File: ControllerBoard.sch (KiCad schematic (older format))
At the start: 1 part, among them U1 nice_nano

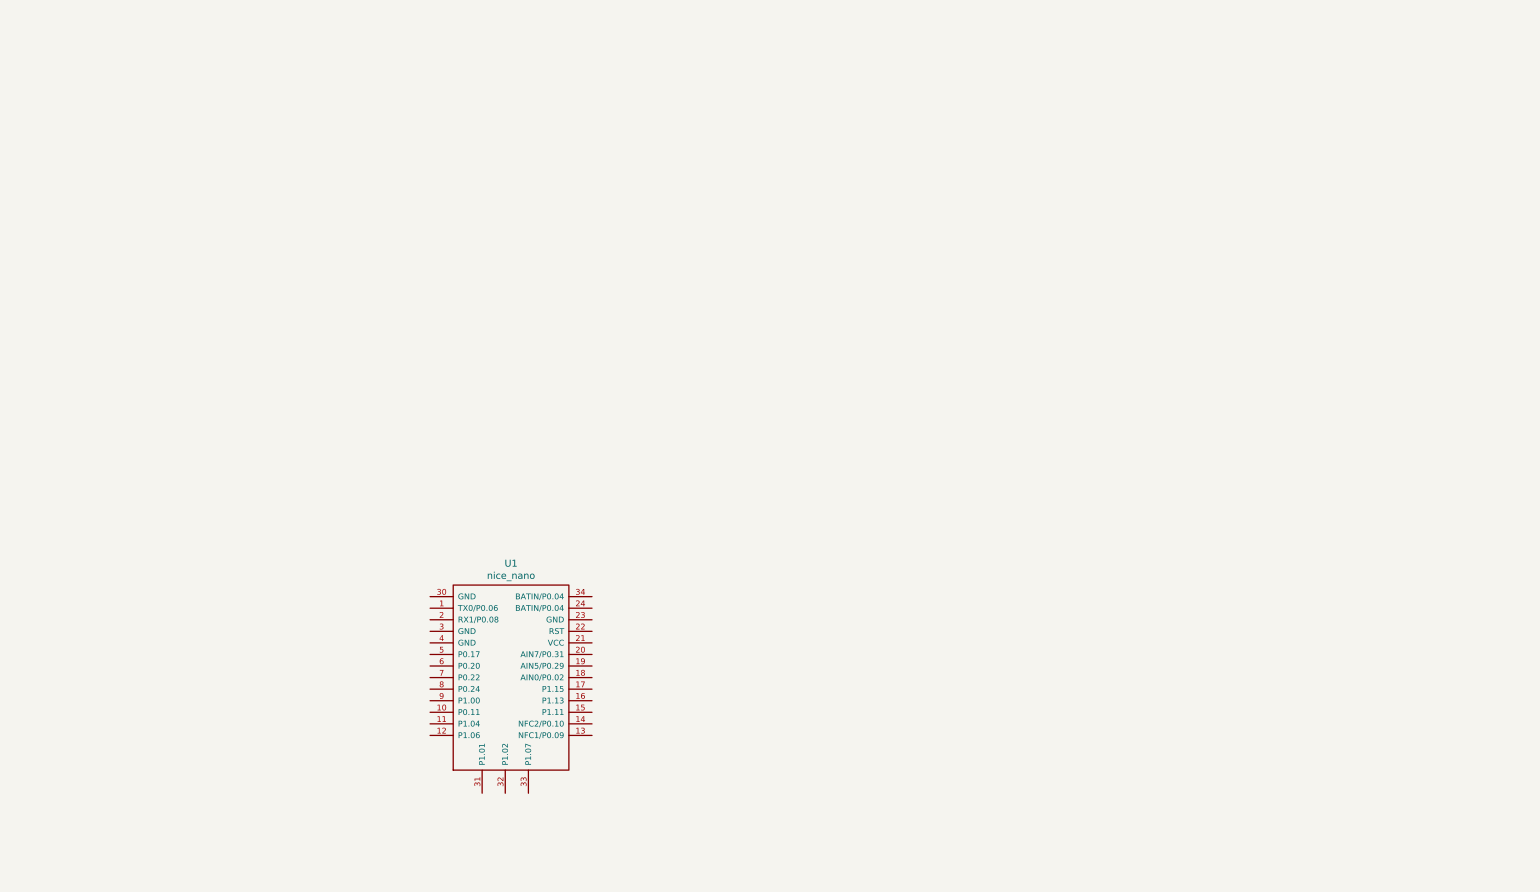
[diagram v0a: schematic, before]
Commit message: First Pass at Wiring
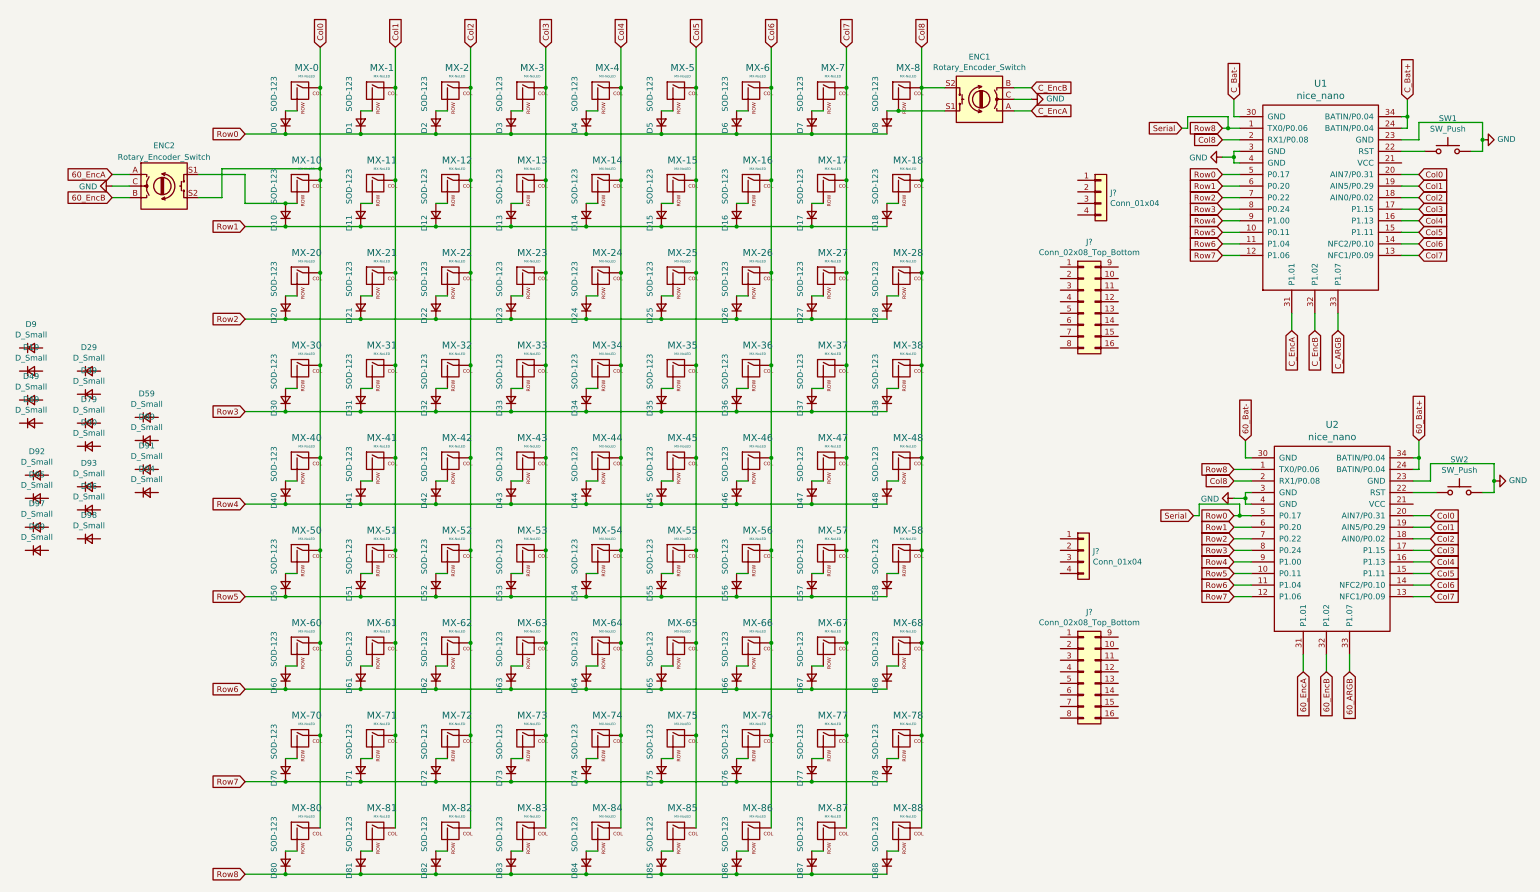
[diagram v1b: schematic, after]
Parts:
- added D0, D1, D10, D11, D12, D13, D14, D15, D16, D17, D18, D2, D20, D21, D22, D23, D24, D25, D26, D27, D28, D3, D30, D31, D32, D33, D34, D35, D36, D37, D38, D4, D40, D41, D42, D43, D44, D45, D46, D47, D48, D5, D50, D51, D52, D53, D54, D55, D56, D57, D58, D6, D60, D61, D62, D63, D64, D65, D66, D67, D68, D7, D70, D71, D72, D73, D74, D75, D76, D77, D78, D8, D80, D81, D82, D83, D84, D85, D86, D87, D88: SOD-123, Keebio-Parts:Diode-Hybrid-Back, symbol Device:D_Small
- added D19, D29, D39, D49, D59, D69, D79, D89, D9, D90, D91, D92, D93, D94, D95, D96, D97, D98, D99: D_Small, symbol Device:D_Small
- added ENC1, ENC2: Rotary_Encoder_Switch, Keebio-Parts:RotaryEncoder_EC11, symbol Device:Rotary_Encoder_Switch
- added J? (x2): Conn_02x08_Top_Bottom, symbol Connector_Generic:Conn_02x08_Top_Bottom
- added J? (x2): Conn_01x04, symbol Connector_Generic:Conn_01x04
- added MX-0, MX-1, MX-10, MX-11, MX-12, MX-13, MX-14, MX-15, MX-16, MX-17, MX-18, MX-2, MX-21, MX-22, MX-23, MX-24, MX-25, MX-26, MX-27, MX-28, MX-3, MX-31, MX-32, MX-33, MX-34, MX-35, MX-36, MX-37, MX-38, MX-4, MX-41, MX-42, MX-43, MX-44, MX-45, MX-46, MX-47, MX-48, MX-5, MX-57, MX-58, MX-6, MX-60, MX-61, MX-62, MX-63, MX-64, MX-65, MX-66, MX-67, MX-68, MX-7, MX-70, MX-71, MX-72, MX-73, MX-74, MX-75, MX-76, MX-77, MX-78, MX-8, MX-80, MX-81, MX-82, MX-83, MX-84, MX-85, MX-86, MX-87, MX-88: MX-NoLED, MX_Alps_Hybrid:MX-1U-NoLED, symbol MX_Alps_Hybrid:MX-NoLED
- added MX-20: MX-NoLED, MX_Alps_Hybrid:MX-1.5U-NoLED, symbol MX_Alps_Hybrid:MX-NoLED
- added MX-30: MX-NoLED, MX_Alps_Hybrid:MX-1.75U-NoLED, symbol MX_Alps_Hybrid:MX-NoLED
- added MX-40: MX-NoLED, MX_Alps_Hybrid:MX-2.25U-NoLED, symbol MX_Alps_Hybrid:MX-NoLED
- added MX-50, MX-51, MX-52, MX-54, MX-55, MX-56: MX-NoLED, MX_Alps_Hybrid:MX-1.25U-NoLED, symbol MX_Alps_Hybrid:MX-NoLED
- added MX-53: MX-NoLED, MX_Alps_Hybrid:MX-6.25U-NoLED, symbol MX_Alps_Hybrid:MX-NoLED
- added SW1, SW2: SW_Push, random-keyboard-parts:SKQG-1155865, symbol Switch:SW_Push
- added U2: nice_nano, nice-nano-kicad:nice_nano, symbol nice_nano:nice_nano
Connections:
- net Row0: now reaches U1.1 (TX0/P0.06)
- net Row0: now also U1.5 (P0.17), D0.1 (K), D1.1 (K), D2.1 (K), D3.1 (K), D4.1 (K), D5.1 (K), D6.1 (K), D7.1 (K), D8.1 (K), D80.1 (K), D81.1 (K), D82.1 (K), D83.1 (K), D84.1 (K), D85.1 (K), D86.1 (K), D87.1 (K), D88.1 (K), U2.1 (TX0/P0.06), U2.5 (P0.17)
- net Row5: now reaches U1.10 (P0.11)
- net Row5: now also D50.1 (K), D51.1 (K), D52.1 (K), D53.1 (K), D54.1 (K), D55.1 (K), D56.1 (K), D57.1 (K), D58.1 (K), U2.10 (P0.11)
- net Row6: now reaches U1.11 (P1.04)
- net Row6: now also D60.1 (K), D61.1 (K), D62.1 (K), D63.1 (K), D64.1 (K), D65.1 (K), D66.1 (K), D67.1 (K), D68.1 (K), U2.11 (P1.04)
- net Row7: now reaches U1.12 (P1.06)
- net Row7: now also D70.1 (K), D71.1 (K), D72.1 (K), D73.1 (K), D74.1 (K), D75.1 (K), D76.1 (K), D77.1 (K), D78.1 (K), U2.12 (P1.06)
- net Col7: now reaches U1.13 (NFC1/P0.09)
- net Col7: now also MX-17.1 (COL), MX-27.1 (COL), MX-37.1 (COL), MX-47.1 (COL), MX-57.1 (COL), MX-67.1 (COL), MX-7.1 (COL), MX-77.1 (COL), MX-87.1 (COL), U2.13 (NFC1/P0.09)
- net Col6: now reaches U1.14 (NFC2/P0.10)
- net Col6: now also MX-16.1 (COL), MX-26.1 (COL), MX-36.1 (COL), MX-46.1 (COL), MX-56.1 (COL), MX-6.1 (COL), MX-66.1 (COL), MX-76.1 (COL), MX-86.1 (COL), U2.14 (NFC2/P0.10)
- net Col5: now reaches U1.15 (P1.11)
- net Col5: now also MX-15.1 (COL), MX-25.1 (COL), MX-35.1 (COL), MX-45.1 (COL), MX-5.1 (COL), MX-55.1 (COL), MX-65.1 (COL), MX-75.1 (COL), MX-85.1 (COL), U2.15 (P1.11)
- net Col4: now reaches U1.16 (P1.13)
- net Col4: now also MX-14.1 (COL), MX-24.1 (COL), MX-34.1 (COL), MX-4.1 (COL), MX-44.1 (COL), MX-54.1 (COL), MX-64.1 (COL), MX-74.1 (COL), MX-84.1 (COL), U2.16 (P1.13)
- net Col3: now reaches U1.17 (P1.15)
- net Col3: now also MX-13.1 (COL), MX-23.1 (COL), MX-3.1 (COL), MX-33.1 (COL), MX-43.1 (COL), MX-53.1 (COL), MX-63.1 (COL), MX-73.1 (COL), MX-83.1 (COL), U2.17 (P1.15)
- net Col2: now reaches U1.18 (AIN0/P0.02)
- net Col2: now also MX-12.1 (COL), MX-2.1 (COL), MX-22.1 (COL), MX-32.1 (COL), MX-42.1 (COL), MX-52.1 (COL), MX-62.1 (COL), MX-72.1 (COL), MX-82.1 (COL), U2.18 (AIN0/P0.02)
- net Col1: now reaches U1.19 (AIN5/P0.29)
- net Col1: now also MX-1.1 (COL), MX-11.1 (COL), MX-21.1 (COL), MX-31.1 (COL), MX-41.1 (COL), MX-51.1 (COL), MX-61.1 (COL), MX-71.1 (COL), MX-81.1 (COL), U2.19 (AIN5/P0.29)
- net Col8: now reaches U1.2 (RX1/P0.08)
- net Col8: now also ENC1.S2, MX-18.1 (COL), MX-28.1 (COL), MX-38.1 (COL), MX-48.1 (COL), MX-58.1 (COL), MX-68.1 (COL), MX-78.1 (COL), MX-8.1 (COL), MX-88.1 (COL), U2.2 (RX1/P0.08)
- net Col0: now reaches U1.20 (AIN7/P0.31)
- net Col0: now also ENC2.S2, MX-0.1 (COL), MX-10.1 (COL), MX-20.1 (COL), MX-30.1 (COL), MX-40.1 (COL), MX-50.1 (COL), MX-60.1 (COL), MX-70.1 (COL), MX-80.1 (COL), U2.20 (AIN7/P0.31)
- net at U1.22 (RST): now also SW1.1
- net GND: now reaches U1.23 (GND)
- net GND: now also U1.3 (GND), U1.4 (GND), ENC1.C, ENC2.C, SW1.2, SW2.2, U2.23 (GND), U2.3 (GND), U2.4 (GND)
- net C_Bat+: now reaches U1.24 (BATIN/P0.04)
- net C_Bat+: now also U1.34 (BATIN/P0.04)
- net C_Bat-: now reaches U1.30 (GND)
- net C_EncA: now reaches U1.31 (P1.01)
- net C_EncA: now also ENC1.A
- net C_EncB: now reaches U1.32 (P1.02)
- net C_EncB: now also ENC1.B
- net C_ARGB: now reaches U1.33 (P1.07)
- net Row1: now reaches U1.6 (P0.20)
- net Row1: now also D10.1 (K), D11.1 (K), D12.1 (K), D13.1 (K), D14.1 (K), D15.1 (K), D16.1 (K), D17.1 (K), D18.1 (K), U2.6 (P0.20)
- net Row2: now reaches U1.7 (P0.22)
- net Row2: now also D20.1 (K), D21.1 (K), D22.1 (K), D23.1 (K), D24.1 (K), D25.1 (K), D26.1 (K), D27.1 (K), D28.1 (K), U2.7 (P0.22)
- net Row3: now reaches U1.8 (P0.24)
- net Row3: now also D30.1 (K), D31.1 (K), D32.1 (K), D33.1 (K), D34.1 (K), D35.1 (K), D36.1 (K), D37.1 (K), D38.1 (K), U2.8 (P0.24)
- net Row4: now reaches U1.9 (P1.00)
- net Row4: now also D40.1 (K), D41.1 (K), D42.1 (K), D43.1 (K), D44.1 (K), D45.1 (K), D46.1 (K), D47.1 (K), D48.1 (K), U2.9 (P1.00)
- new net: D16.2 (A), MX-16.2 (ROW)
- new net: D17.2 (A), MX-17.2 (ROW)
- new net: D18.2 (A), MX-18.2 (ROW)
- new net: D10.2 (A), ENC2.S1, MX-10.2 (ROW)
- new net: D11.2 (A), MX-11.2 (ROW)
- new net: D12.2 (A), MX-12.2 (ROW)
- new net: D13.2 (A), MX-13.2 (ROW)
- new net: D14.2 (A), MX-14.2 (ROW)
- new net: D15.2 (A), MX-15.2 (ROW)
- new net: D26.2 (A), MX-26.2 (ROW)
- new net: D27.2 (A), MX-27.2 (ROW)
- new net: D28.2 (A), MX-28.2 (ROW)
- new net: D20.2 (A), MX-20.2 (ROW)
- new net: D21.2 (A), MX-21.2 (ROW)
- new net: D22.2 (A), MX-22.2 (ROW)
- new net: D23.2 (A), MX-23.2 (ROW)
- new net: D24.2 (A), MX-24.2 (ROW)
- new net: D25.2 (A), MX-25.2 (ROW)
- new net: D36.2 (A), MX-36.2 (ROW)
- new net: D37.2 (A), MX-37.2 (ROW)
- new net: D38.2 (A), MX-38.2 (ROW)
- new net: D30.2 (A), MX-30.2 (ROW)
- new net: D31.2 (A), MX-31.2 (ROW)
- new net: D32.2 (A), MX-32.2 (ROW)
- new net: D33.2 (A), MX-33.2 (ROW)
- new net: D34.2 (A), MX-34.2 (ROW)
- new net: D35.2 (A), MX-35.2 (ROW)
- new net: D46.2 (A), MX-46.2 (ROW)
- new net: D47.2 (A), MX-47.2 (ROW)
- new net: D48.2 (A), MX-48.2 (ROW)
- new net: D40.2 (A), MX-40.2 (ROW)
- new net: D41.2 (A), MX-41.2 (ROW)
- new net: D42.2 (A), MX-42.2 (ROW)
- new net: D43.2 (A), MX-43.2 (ROW)
- new net: D44.2 (A), MX-44.2 (ROW)
- new net: D45.2 (A), MX-45.2 (ROW)
- new net: D56.2 (A), MX-56.2 (ROW)
- new net: D57.2 (A), MX-57.2 (ROW)
- new net: D58.2 (A), MX-58.2 (ROW)
- new net: D50.2 (A), MX-50.2 (ROW)
- new net: D51.2 (A), MX-51.2 (ROW)
- new net: D52.2 (A), MX-52.2 (ROW)
- new net: D53.2 (A), MX-53.2 (ROW)
- new net: D54.2 (A), MX-54.2 (ROW)
- new net: D55.2 (A), MX-55.2 (ROW)
- new net: D66.2 (A), MX-66.2 (ROW)
- new net: D67.2 (A), MX-67.2 (ROW)
- new net: D68.2 (A), MX-68.2 (ROW)
- new net: D60.2 (A), MX-60.2 (ROW)
- new net: D61.2 (A), MX-61.2 (ROW)
- new net: D62.2 (A), MX-62.2 (ROW)
- new net: D63.2 (A), MX-63.2 (ROW)
- new net: D64.2 (A), MX-64.2 (ROW)
- new net: D65.2 (A), MX-65.2 (ROW)
- new net: D76.2 (A), MX-76.2 (ROW)
- new net: D77.2 (A), MX-77.2 (ROW)
- new net: D78.2 (A), MX-78.2 (ROW)
- new net: D70.2 (A), MX-70.2 (ROW)
- new net: D71.2 (A), MX-71.2 (ROW)
- new net: D72.2 (A), MX-72.2 (ROW)
- new net: D73.2 (A), MX-73.2 (ROW)
- new net: D74.2 (A), MX-74.2 (ROW)
- new net: D75.2 (A), MX-75.2 (ROW)
- new net: D86.2 (A), MX-86.2 (ROW)
- new net: D87.2 (A), MX-87.2 (ROW)
- new net: D88.2 (A), MX-88.2 (ROW)
- new net: D80.2 (A), MX-80.2 (ROW)
- new net: D81.2 (A), MX-81.2 (ROW)
- new net: D82.2 (A), MX-82.2 (ROW)
- new net: D83.2 (A), MX-83.2 (ROW)
- new net: D84.2 (A), MX-84.2 (ROW)
- new net: D85.2 (A), MX-85.2 (ROW)
- new net: D6.2 (A), MX-6.2 (ROW)
- new net: D7.2 (A), MX-7.2 (ROW)
- new net: D8.2 (A), ENC1.S1, MX-8.2 (ROW)
- new net: D0.2 (A), MX-0.2 (ROW)
- new net: D1.2 (A), MX-1.2 (ROW)
- new net: D2.2 (A), MX-2.2 (ROW)
- new net: D3.2 (A), MX-3.2 (ROW)
- new net: D4.2 (A), MX-4.2 (ROW)
- new net: D5.2 (A), MX-5.2 (ROW)
- new net: SW2.1, U2.22 (RST)
- new net 60_ARGB: U2.33 (P1.07)
- new net 60_Bat+: U2.24 (BATIN/P0.04), U2.34 (BATIN/P0.04)
- new net 60_Bat-: U2.30 (GND)
- new net 60_EncA: ENC2.A, U2.31 (P1.01)
- new net 60_EncB: ENC2.B, U2.32 (P1.02)
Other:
- moved on the sheet: U1
